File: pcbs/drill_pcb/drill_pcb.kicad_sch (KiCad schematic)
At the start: 78 parts, among them SW1 RPi reset, SW2 SW_Push, SW3 SW_Push, SW4 SW_Push, U1 PCA9306, U2 Pico, U3 L7805, U4 IFX007T, U5 IFX007T, U6 ACS712xLCTR-20A, U7 HT75xx-1-SOT89

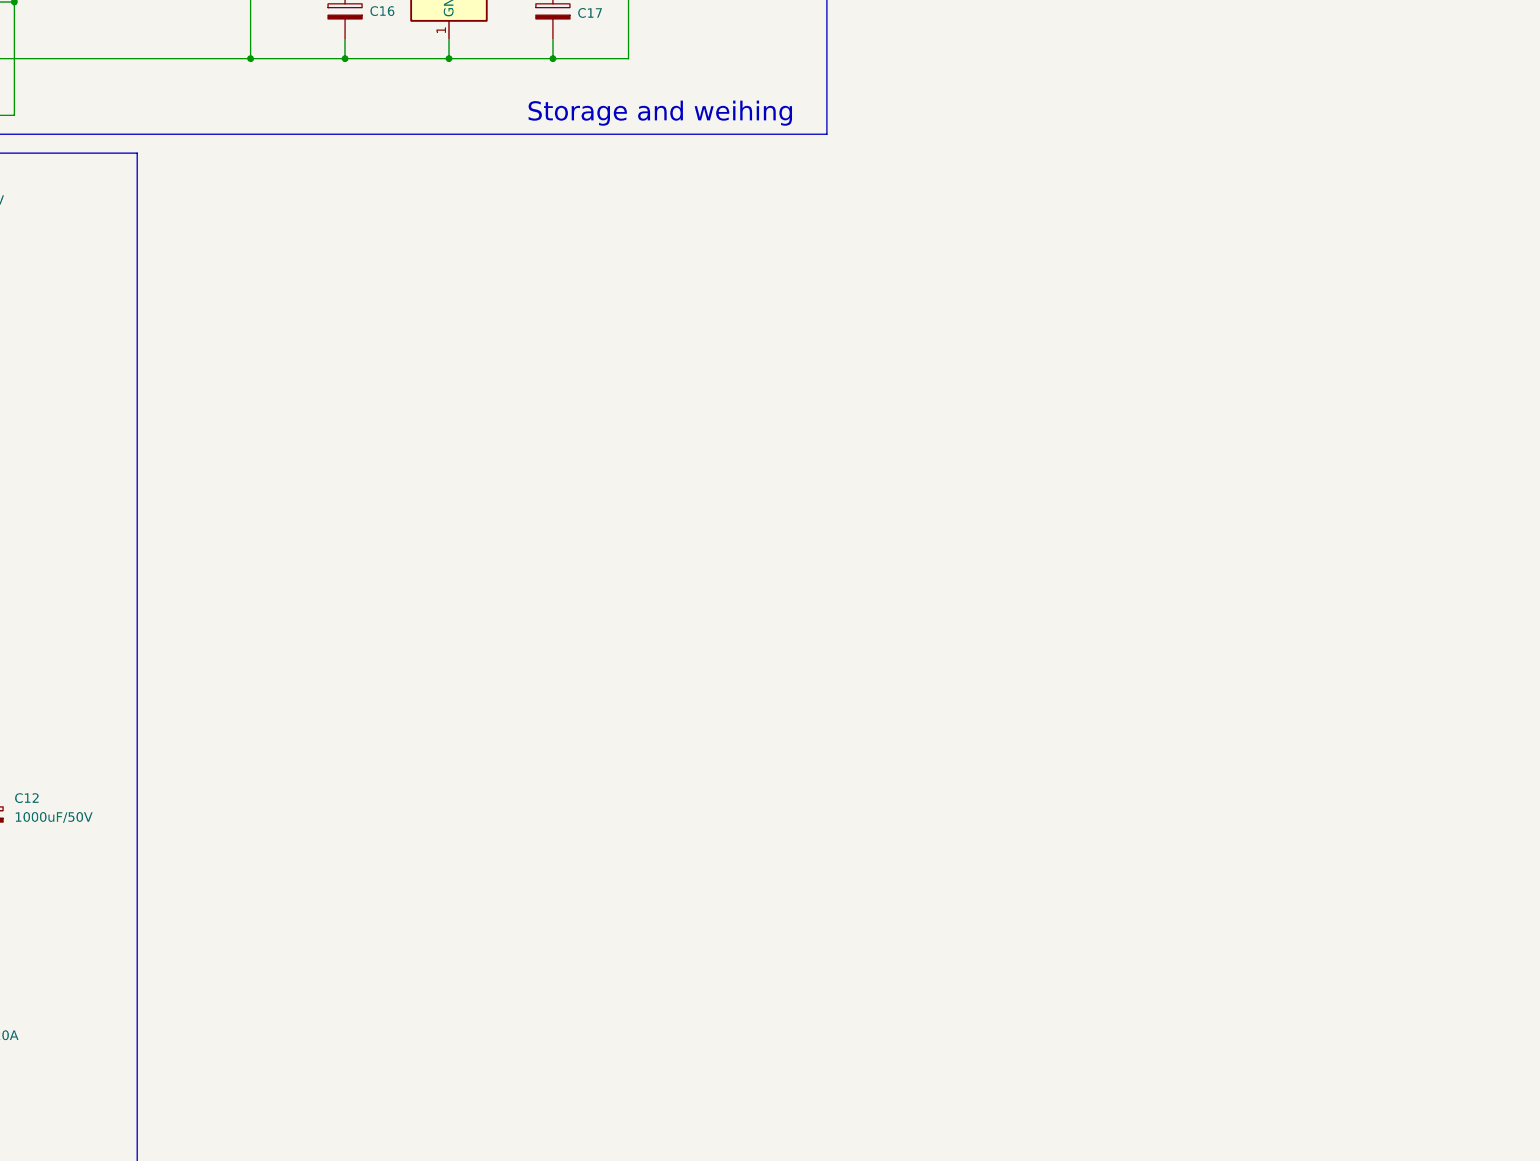
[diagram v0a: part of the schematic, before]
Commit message: pridany_pojezd
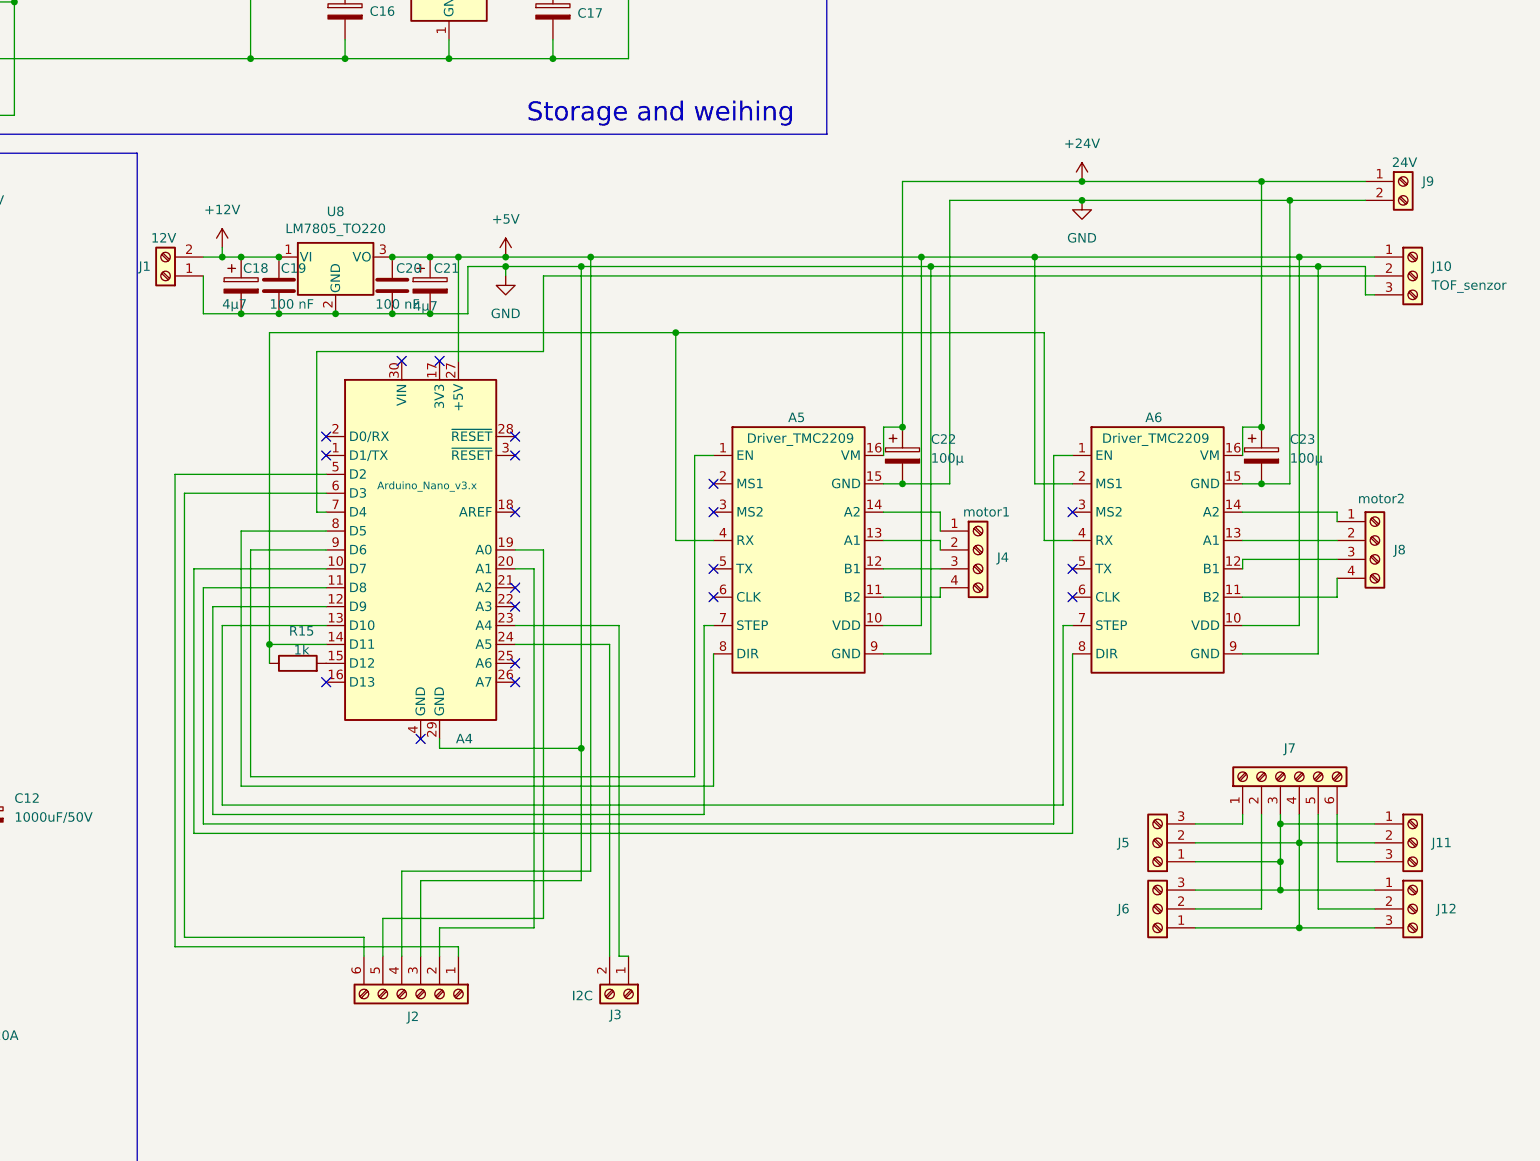
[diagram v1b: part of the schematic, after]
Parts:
- added A4: Arduino_Nano_v3.x, Module:Arduino_Nano, symbol MCU_Module:Arduino_Nano_v3.x
- added A5, A6: Driver_TMC2209, Module:Pololu_Breakout-16_15.2x20.3mm, symbol mujDriver:mujDriver2
- added C18, C21: 4μ7, Capacitor_THT:CP_Radial_D5.0mm_P2.50mm, symbol Device:C_Polarized
- added C19, C20: 100 nF, Capacitor_THT:C_Disc_D4.3mm_W1.9mm_P5.00mm, symbol Device:C
- added C22, C23: 100μ, Capacitor_THT:CP_Radial_D8.0mm_P3.50mm, symbol Device:C_Polarized
- added J1: 12V, Connector_AMASS:AMASS_XT60-M_1x02_P7.20mm_Vertical, symbol Connector:Screw_Terminal_01x02
- added J10: TOF_senzor, Connector_JST:JST_XH_B3B-XH-A_1x03_P2.50mm_Vertical, symbol Connector:Screw_Terminal_01x03
- added J11, J12, J5, J6: Screw_Terminal_01x03, Connector_JST:JST_XH_S3B-XH-A-1_1x03_P2.50mm_Horizontal, symbol Connector:Screw_Terminal_01x03
- added J2: Screw_Terminal_01x06, Connector_JST:JST_XH_B6B-XH-A_1x06_P2.50mm_Vertical, symbol Connector:Screw_Terminal_01x06
- added J3: I2C, Connector_JST:JST_XH_B2B-XH-A_1x02_P2.50mm_Vertical, symbol Connector:Screw_Terminal_01x02
- added J4: motor1, Connector_JST:JST_XH_B4B-XH-A_1x04_P2.50mm_Vertical, symbol Connector:Screw_Terminal_01x04
- added J7: Screw_Terminal_01x06, Connector_JST:JST_XH_S6B-XH-A-1_1x06_P2.50mm_Horizontal, symbol Connector:Screw_Terminal_01x06
- added J8: motor2, Connector_JST:JST_XH_B4B-XH-A_1x04_P2.50mm_Vertical, symbol Connector:Screw_Terminal_01x04
- added J9: 24V, kiCad:DEANS, symbol Connector:Screw_Terminal_01x02
- added R15: 1k, Resistor_SMD:R_1206_3216Metric, symbol Device:R
- added U8: LM7805_TO220, Package_TO_SOT_THT:TO-220-3_Vertical, symbol Regulator_Linear:LM7805_TO220
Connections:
- net +12V: now also C18.1, C19.1, J1.2 (Pin_2), U8.1 (VI)
- net +24V: now also A5.16 (VM), A6.16 (VM), C22.1, C23.1, J9.1 (Pin_1)
- net +5V: now also A4.27 (+5V), A5.10 (VDD), A6.10 (VDD), A6.2 (MS1), C20.1, C21.1, J10.1 (Pin_1), J2.4 (Pin_4), U8.3 (VO)
- net GND: now also A4.29 (GND), A5.15 (GND), A5.9 (GND), A6.15 (GND), A6.9 (GND), C18.2, C19.2, C20.2, C21.2, C22.2, C23.2, J1.1 (Pin_1), J10.3 (Pin_3), J2.3 (Pin_3), J9.2 (Pin_2), U8.2 (GND)
- new net: A4.5 (D2), J2.1 (Pin_1)
- new net: A4.20 (A1), J2.2 (Pin_2)
- new net: A4.19 (A0), J2.5 (Pin_5)
- new net: A4.6 (D3), J2.6 (Pin_6)
- new net: A4.23 (A4), J3.1 (Pin_1)
- new net: A4.24 (A5), J3.2 (Pin_2)
- new net: J11.2 (Pin_2), J12.3 (Pin_3), J5.2 (Pin_2), J6.1 (Pin_1), J7.4 (Pin_4)
- new net: J6.2 (Pin_2), J7.2 (Pin_2)
- new net: J11.1 (Pin_1), J12.1 (Pin_1), J5.1 (Pin_1), J6.3 (Pin_3), J7.3 (Pin_3)
- new net: A4.7 (D4), J10.2 (Pin_2)
- new net: A4.9 (D6), A5.1 (EN)
- new net: A5.11 (B2), J4.4 (Pin_4)
- new net: A5.12 (B1), J4.3 (Pin_3)
- new net: A5.13 (A1), J4.2 (Pin_2)
- new net: A5.14 (A2), J4.1 (Pin_1)
- new net: A4.14 (D11), A5.4 (RX), A6.4 (RX), R15.1
- new net: A4.12 (D9), A5.7 (STEP)
- new net: A4.8 (D5), A5.8 (DIR)
- new net: J5.3 (Pin_3), J7.1 (Pin_1)
- new net: J12.2 (Pin_2), J7.5 (Pin_5)
- new net: J11.3 (Pin_3), J7.6 (Pin_6)
- new net: A4.15 (D12), R15.2
- new net: A4.11 (D8), A6.1 (EN)
- new net: A6.11 (B2), J8.4 (Pin_4)
- new net: A6.12 (B1), J8.3 (Pin_3)
- new net: A6.13 (A1), J8.2 (Pin_2)
- new net: A6.14 (A2), J8.1 (Pin_1)
- new net: A4.13 (D10), A6.7 (STEP)
- new net: A4.10 (D7), A6.8 (DIR)
- no-connect marks 64 -> 84
